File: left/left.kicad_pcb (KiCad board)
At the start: 2 copper layers, 117.6 x 97.9 mm, 53 parts, among them J1 USB_C_Receptacle_IN, J2 USB_C_Receptacle_OUT, SW1 SW_Push, SW2 SW_SPDT, U1 STM32G0B1CBTx, U2 SRV05-4, U3 XC6206P332MR, U4 SRV05-4

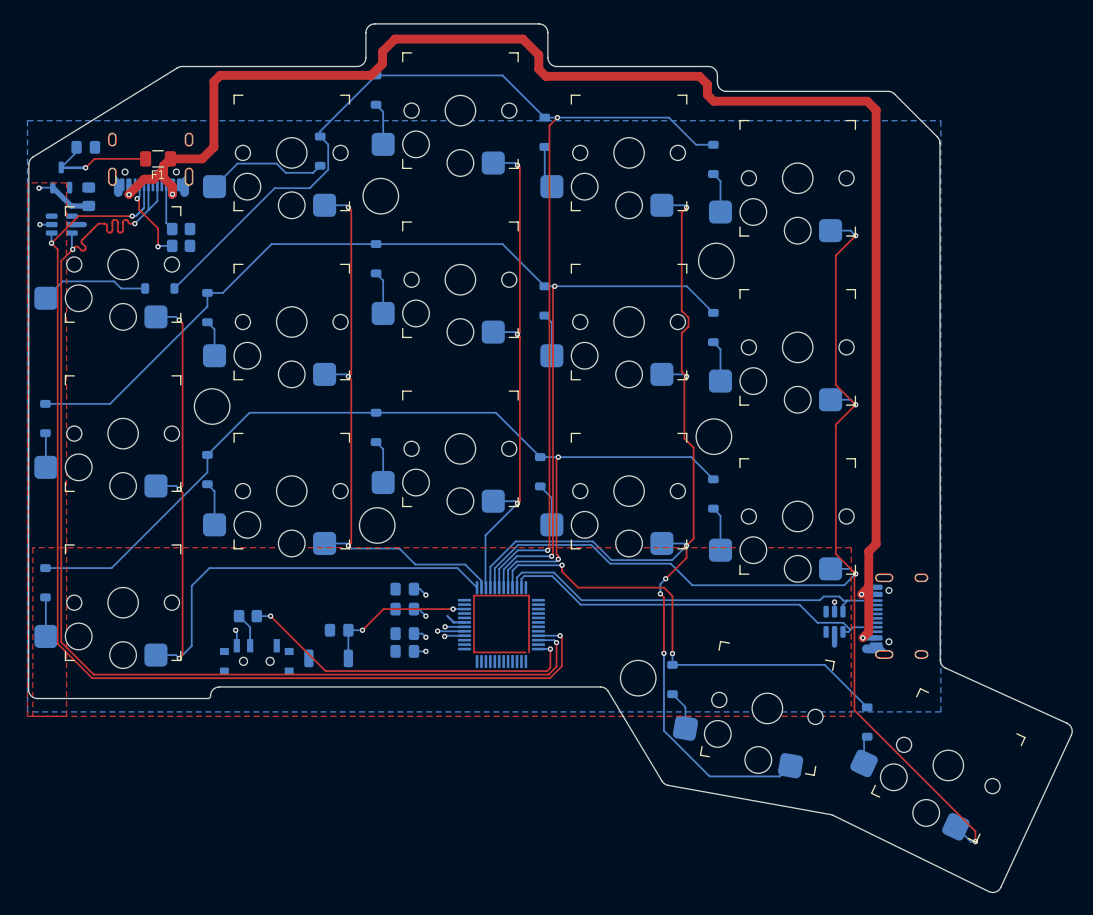
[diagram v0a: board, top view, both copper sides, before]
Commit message: v3 for left
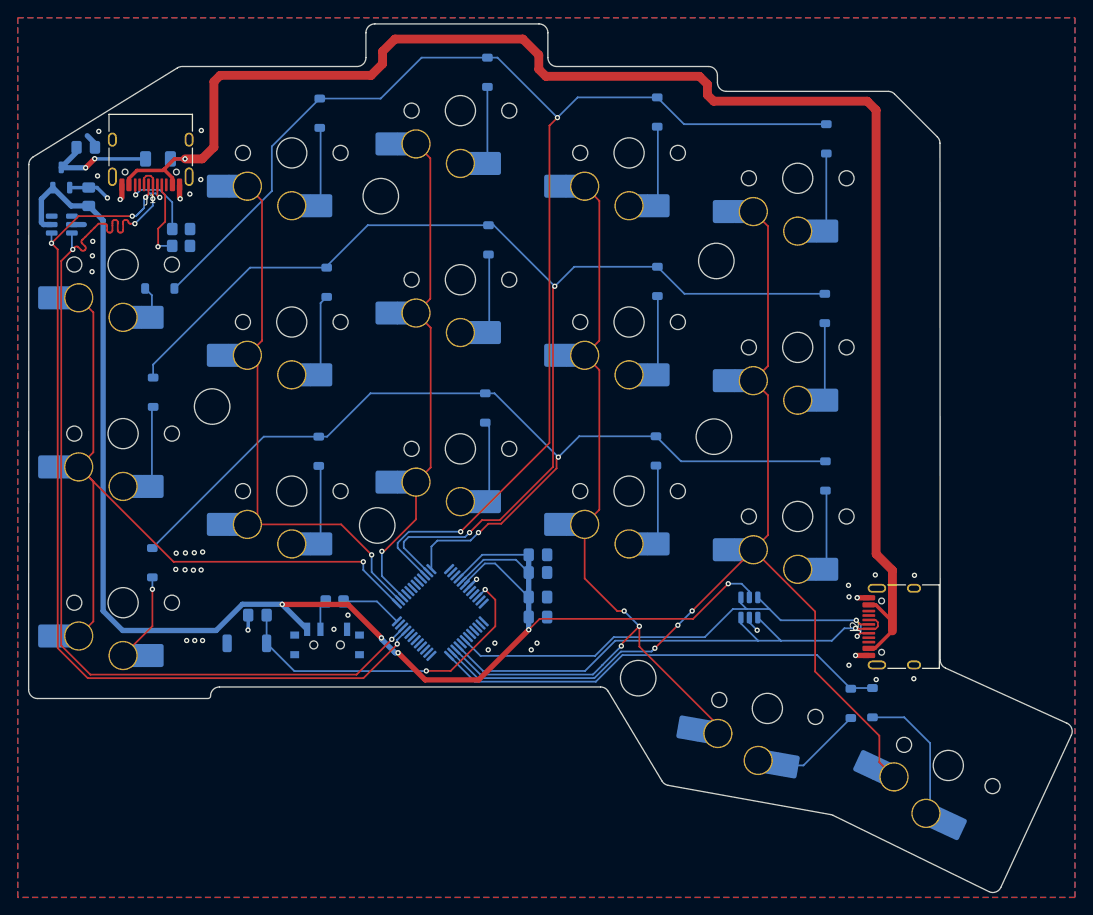
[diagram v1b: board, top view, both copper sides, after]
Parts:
- F1: moved to B.Cu
- J1, J2: moved to F.Cu
- KEY1, KEY10, KEY11, KEY12, KEY13, KEY14, KEY15, KEY16, KEY17, KEY2, KEY3, KEY4, KEY5, KEY6, KEY7, KEY8, KEY9: footprint Low Profile Keyswitches:SW_Kailh_Choc_V1_HotSwap -> Keyswitch Marbastlib Choc:SW_choc_v1_HS_CPG135001S30_1u; moved to B.Cu
- moved D17 20.3 mm to (139.2, 122.5)
- moved C2 18.5 mm to (103.9, 105.8), turned to 0 degrees
- moved C1 16.5 mm to (103.9, 107.8), turned to 0 degrees
- moved C3 15.3 mm to (103.9, 112.8), turned to 0 degrees
- moved C4 15.1 mm to (103.9, 110.6), turned to 0 degrees
- moved D9 13.7 mm to (80.1, 75.1)
- moved D12 13.2 mm to (117.2, 94.1)
- moved D1 12.9 mm to (136.4, 58.9)
- moved D7 12.9 mm to (117.4, 75.0)
- moved D2 12.9 mm to (117.3, 55.9)
- moved D8 12.8 mm to (98.3, 70.3)
- moved D11 12.8 mm to (136.3, 96.9)
- moved D6 12.7 mm to (136.2, 78.0)
- moved D14 12.7 mm to (79.2, 94.1)
- moved D3 12.7 mm to (98.2, 51.4)
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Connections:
- J2 pad A6: unconnected-(J2-D+-PadA6) -> TX
- J2 pad A7: unconnected-(J2-D--PadA7) -> RX
- J2 pad A8: RX -> unconnected-(J2-SBU1-PadA8)
- J2 pad B6: unconnected-(J2-D+-PadB6) -> TX
- J2 pad B7: unconnected-(J2-D--PadB7) -> RX
- J2 pad B8: TX -> unconnected-(J2-SBU2-PadB8)
- U1 pad 13: COL4 -> unconnected-(U1-PA2-Pad13)
- U1 pad 14: COL3 -> unconnected-(U1-PA3-Pad14)
- U1 pad 15: COL2 -> unconnected-(U1-PA4-Pad15)
- U1 pad 16: COL1 -> unconnected-(U1-PA5-Pad16)
- U1 pad 17: COL0 -> unconnected-(U1-PA6-Pad17)
- U1 pad 18: ROW0 -> unconnected-(U1-PA7-Pad18)
- U1 pad 19: ROW1 -> RX
- U1 pad 20: ROW2 -> unconnected-(U1-PB1-Pad20)
- U1 pad 21: ROW3 -> TX
- U1 pad 22: TX -> COL1
- U1 pad 23: RX -> COL0
- U1 pad 24: unconnected-(U1-PB12-Pad24) -> ROW3
- U1 pad 37: unconnected-(U1-PA15-Pad37) -> COL4
- U1 pad 38: unconnected-(U1-PD0-Pad38) -> COL3
- U1 pad 39: unconnected-(U1-PD1-Pad39) -> COL2
- U1 pad 46: unconnected-(U1-PB7-Pad46) -> ROW0
- U1 pad 47: unconnected-(U1-PB8-Pad47) -> ROW1
- U1 pad 48: unconnected-(U1-PB9-Pad48) -> ROW2
- U2 pad 1: RX -> TX
- U2 pad 3: unconnected-(U2-IO2-Pad3) -> TX
- U2 pad 4: unconnected-(U2-IO3-Pad4) -> RX
- U2 pad 6: TX -> RX
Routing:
- net +3.3V: track 24.3 -> 181.4 mm, vias 11 -> 5
- net BOOT0: track 39.3 -> 6.94 mm, vias 2 -> 0
- net (no net): track 24.8 -> 0.00 mm
- net COL0: track 136.1 -> 114.1 mm, vias 4 -> 3
- net nRST: track 17.3 -> 38.4 mm
- net ROW0: track 135.3 -> 155.9 mm
- net D-: track 130.1 -> 109.7 mm, vias 3 -> 5
- net D+: track 131.8 -> 111.5 mm, vias 3 -> 4
- net COL1: track 115.1 -> 95.7 mm, vias 6 -> 3
- net TX: track 45.0 -> 59.3 mm, vias 0 -> 1
- net Net-(D16-A): track 3.15 -> 16.6 mm
- net RX: track 44.7 -> 56.5 mm, vias 0 -> 2
- net Net-(D5-A): track 12.3 -> 3.57 mm
- net ROW1: track 125.5 -> 134.1 mm
- net GND: track 12.1 -> 19.2 mm, vias 0 -> 40
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- added copper zone on F.Cu, net GND
- removed copper zone on F.Cu, net +3.3V
